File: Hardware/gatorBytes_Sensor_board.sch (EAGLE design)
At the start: 24 parts, among them U2 LIGHT_SENSORTEMT6000, U3 MCP9700TT

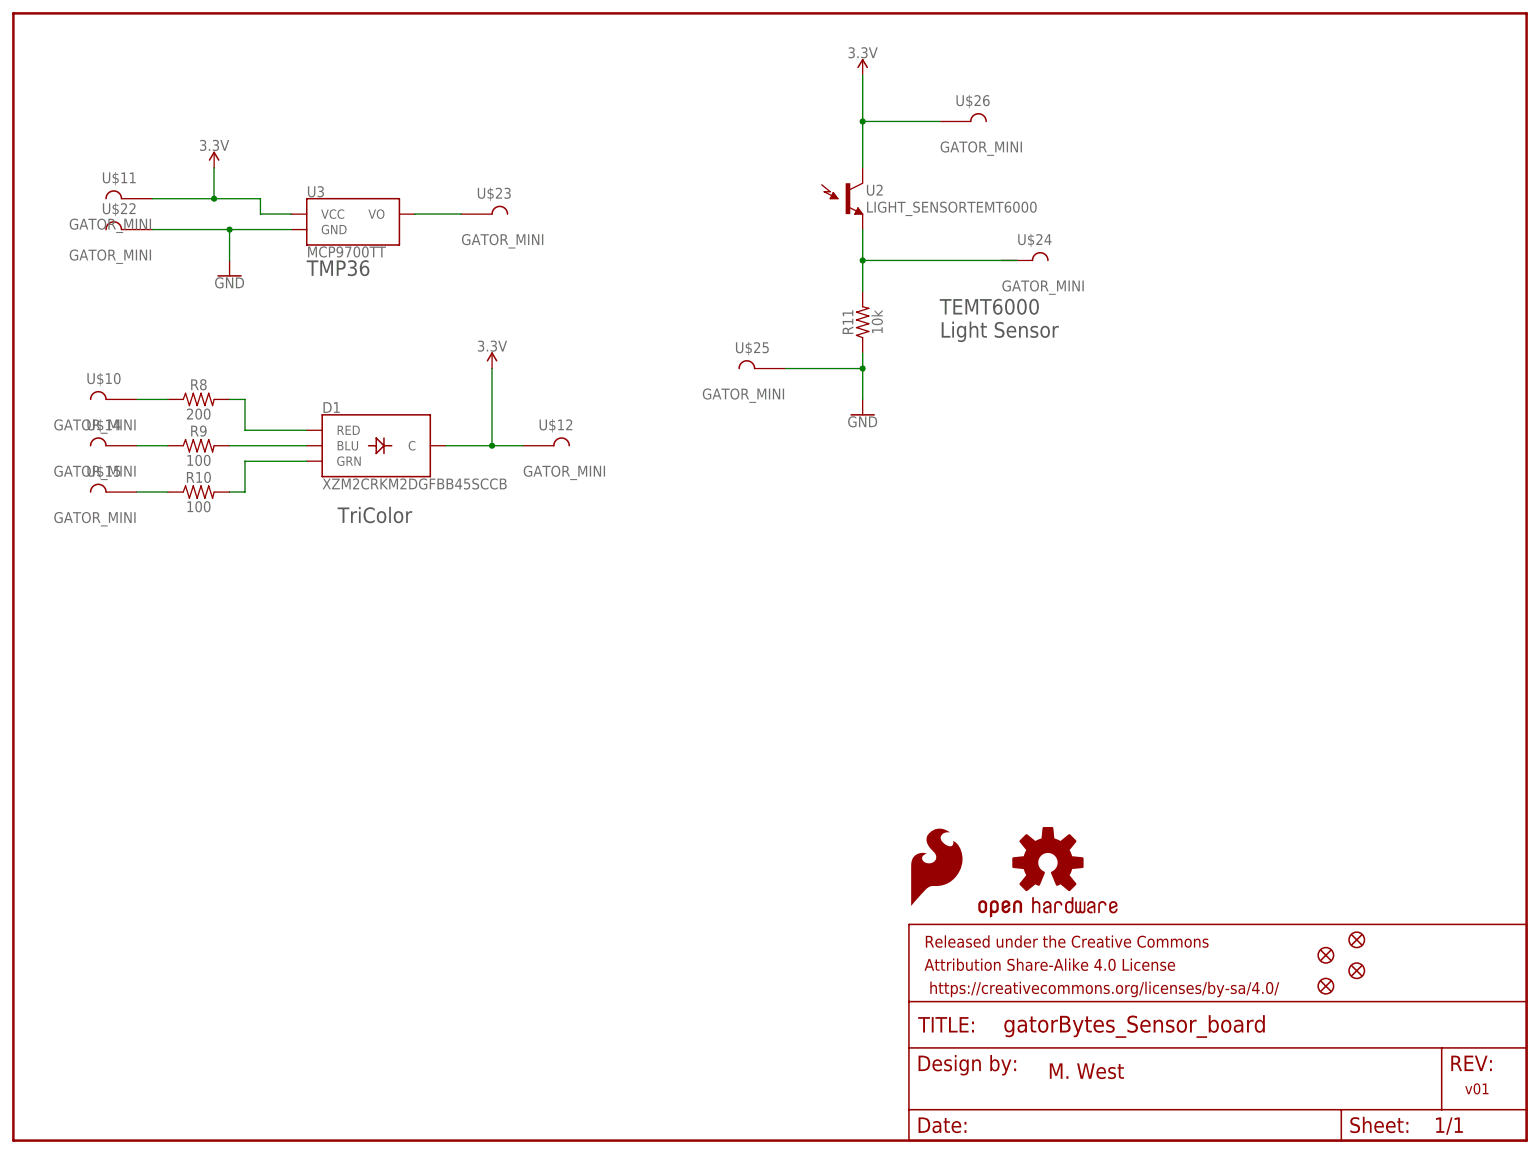
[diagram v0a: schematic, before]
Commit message: adding new tabs
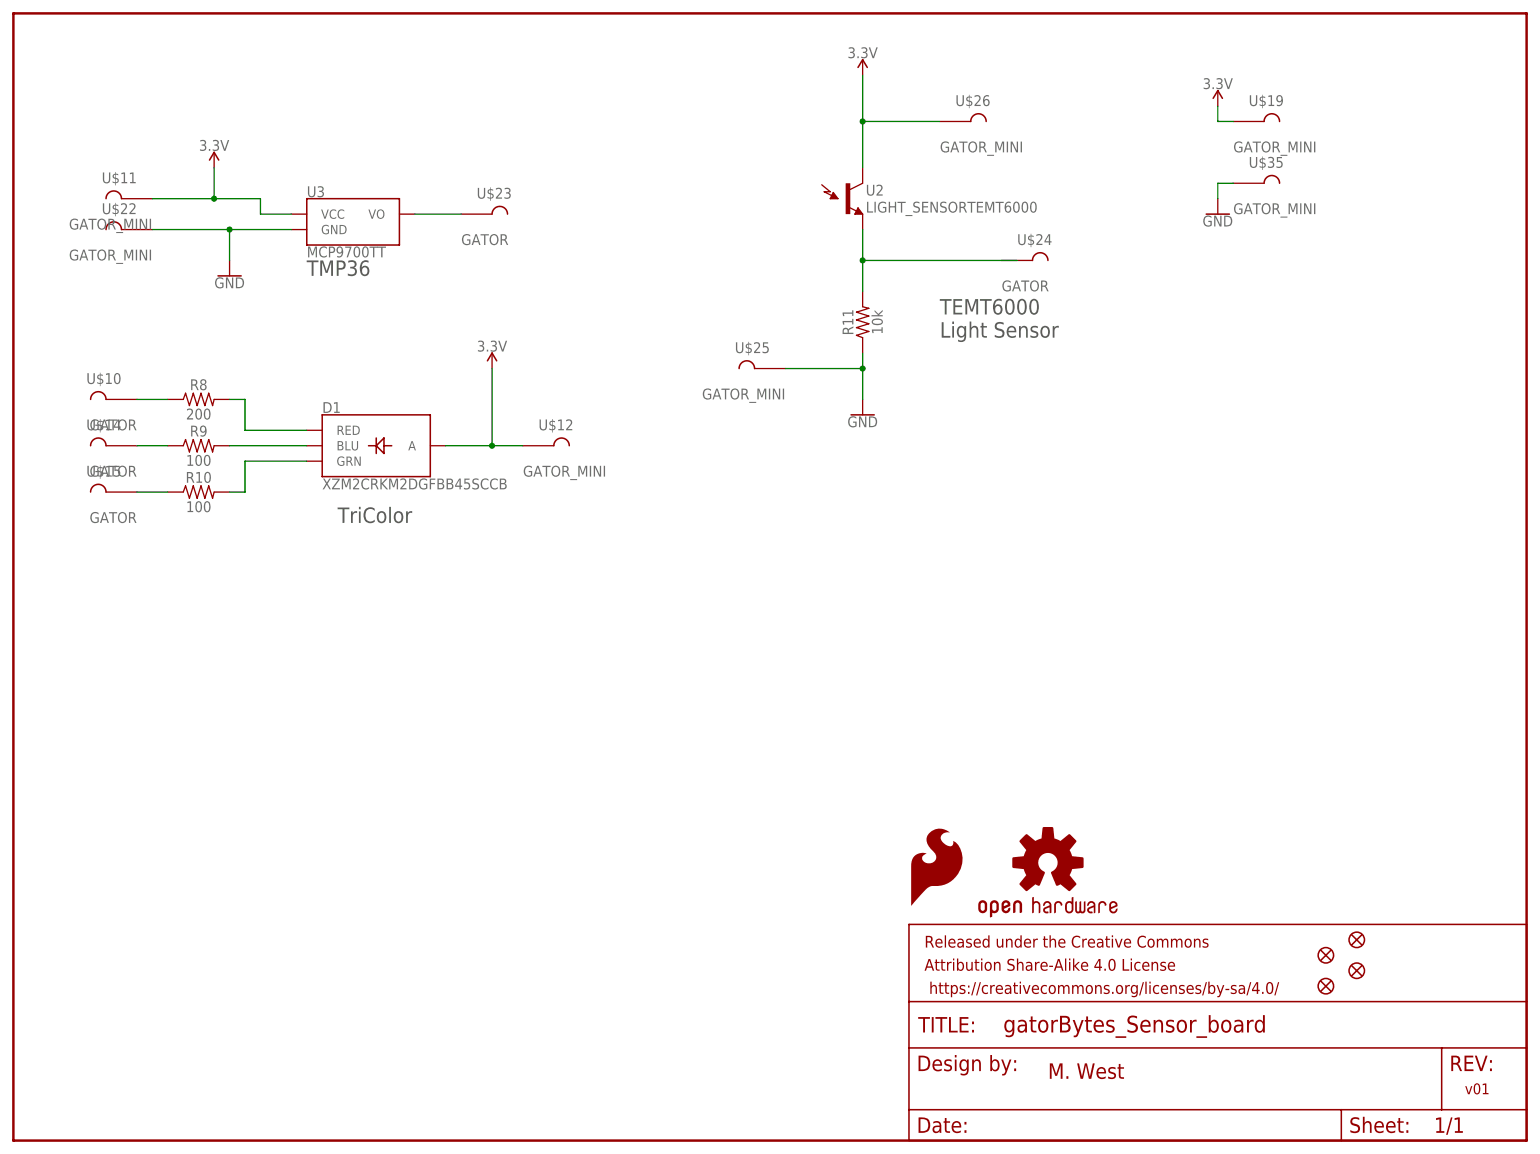
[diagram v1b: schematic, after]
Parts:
- added U$19, U$35: GATOR_MINI, TAB:GATOR_MINI
- D1: device SparkFun-LED:SUNLEDSMD1 -> SparkFun-LED:LED-RGB-CASMD
- U$10, U$14, U$15, U$23, U$24: value GATOR_MINI -> GATOR; device TAB:GATOR_MINI -> SparkFun-Connectors:GATOR
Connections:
- net 3.3V: now also D1.A, U$19.P$1; no longer D1.C
- net GND: now also U$35.P$1

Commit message: post checklist chanegs
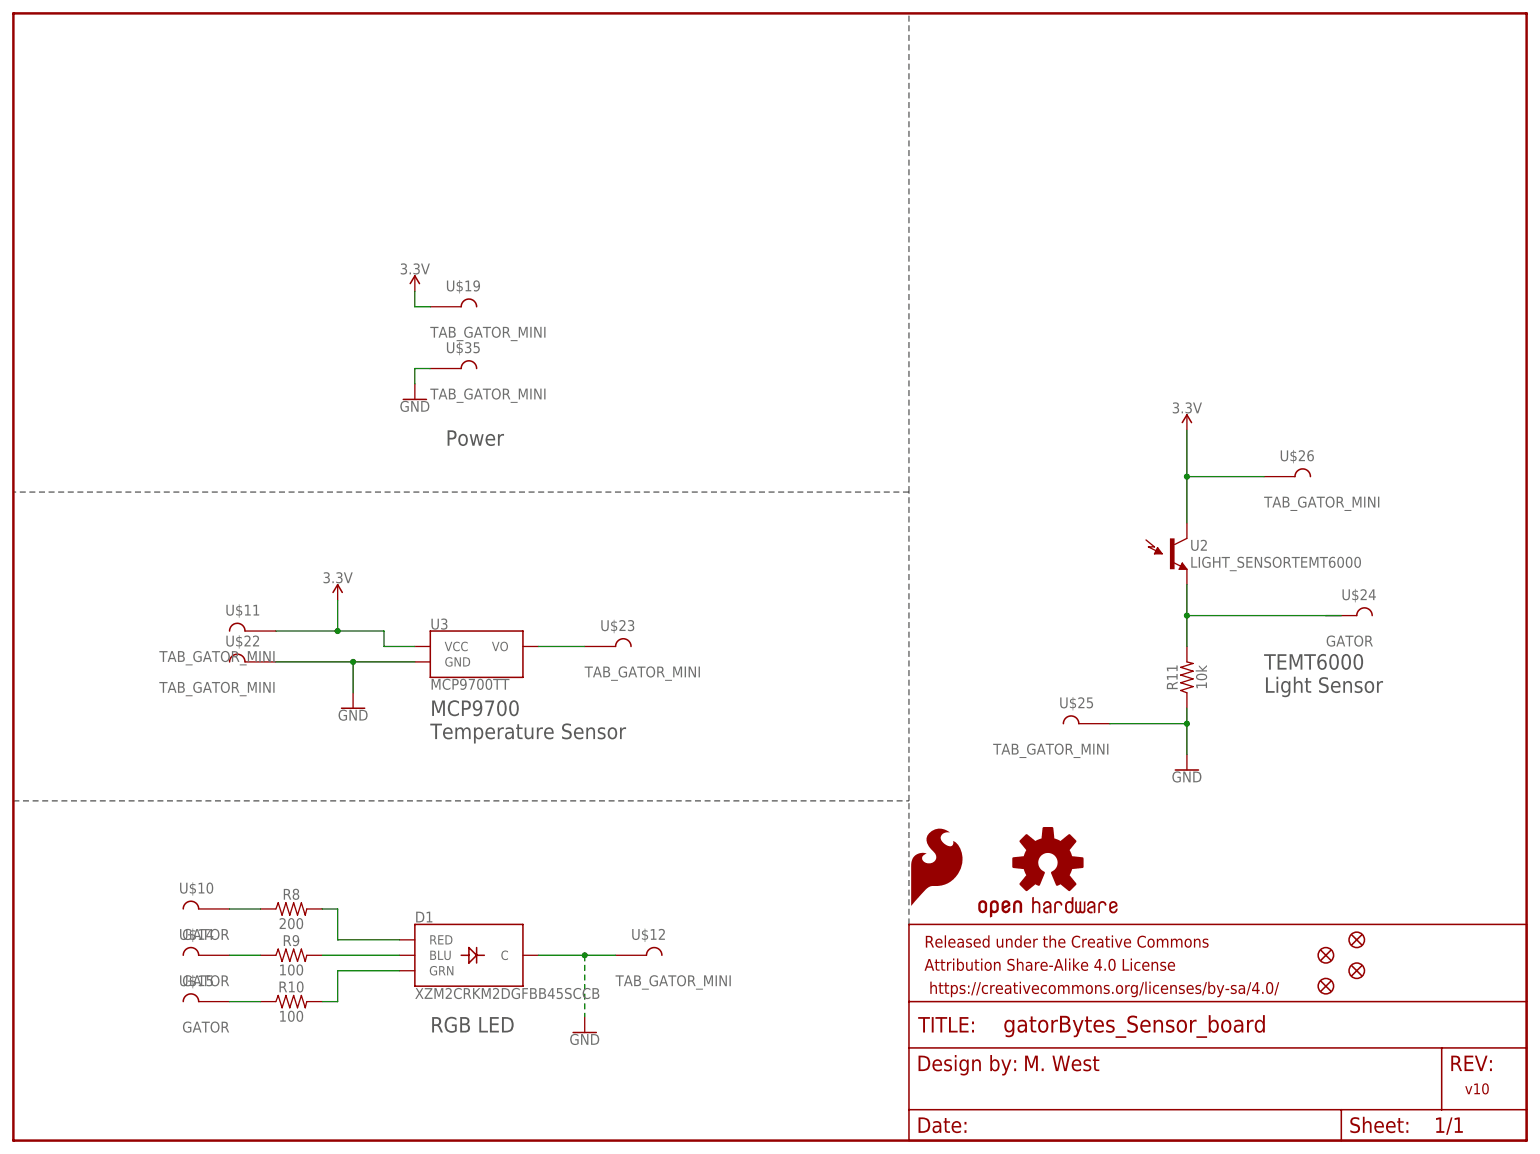
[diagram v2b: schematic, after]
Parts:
- D1: device SparkFun-LED:LED-RGB-CASMD -> SparkFun-LED:SUNLEDSMD1
- U$11, U$12, U$19, U$22, U$25, U$26, U$35: value GATOR_MINI -> TAB_GATOR_MINI; device TAB:GATOR_MINI -> SparkFun-Connectors:TAB_GATOR_MINI
- U$23: value GATOR -> TAB_GATOR_MINI; device SparkFun-Connectors:GATOR -> SparkFun-Connectors:TAB_GATOR_MINI
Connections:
- net 3.3V: no longer D1.A, U$12.P$1
- net GND: now also D1.C, U$12.P$1
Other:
- note added: "MCP9700 Temperature Sensor"
- note added: "Power"
- note added: "RGB LED"
- note added: "v10"
- note removed: "TMP36"
- note removed: "TriColor"
- note removed: "v01"
- moved on the sheet: R10, R11, R8, R9, U$10, U$11, U$12, U$14, U$15, U$19, U$22, U$23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
